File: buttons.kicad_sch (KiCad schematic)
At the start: 21 parts, among them SW1 SW_SPST, SW10 SW_SPST, SW11 SW_SPST, SW12 SW_SPST, SW13 SW_SPST, SW14 SW_SPST, SW15 SW_SPST, SW16 SW_SPST, SW17 SW_SPST, SW18 SW_SPST, SW19 SW_SPST, SW2 SW_SPST, SW20 SW_SPST, SW3 SW_SPST, SW4 SW_SPST, SW5 SW_SPST, SW6 SW_SPST, SW7 SW_SPST, SW8 SW_SPST, SW9 SW_SPST, U3 CD74HC4067M96

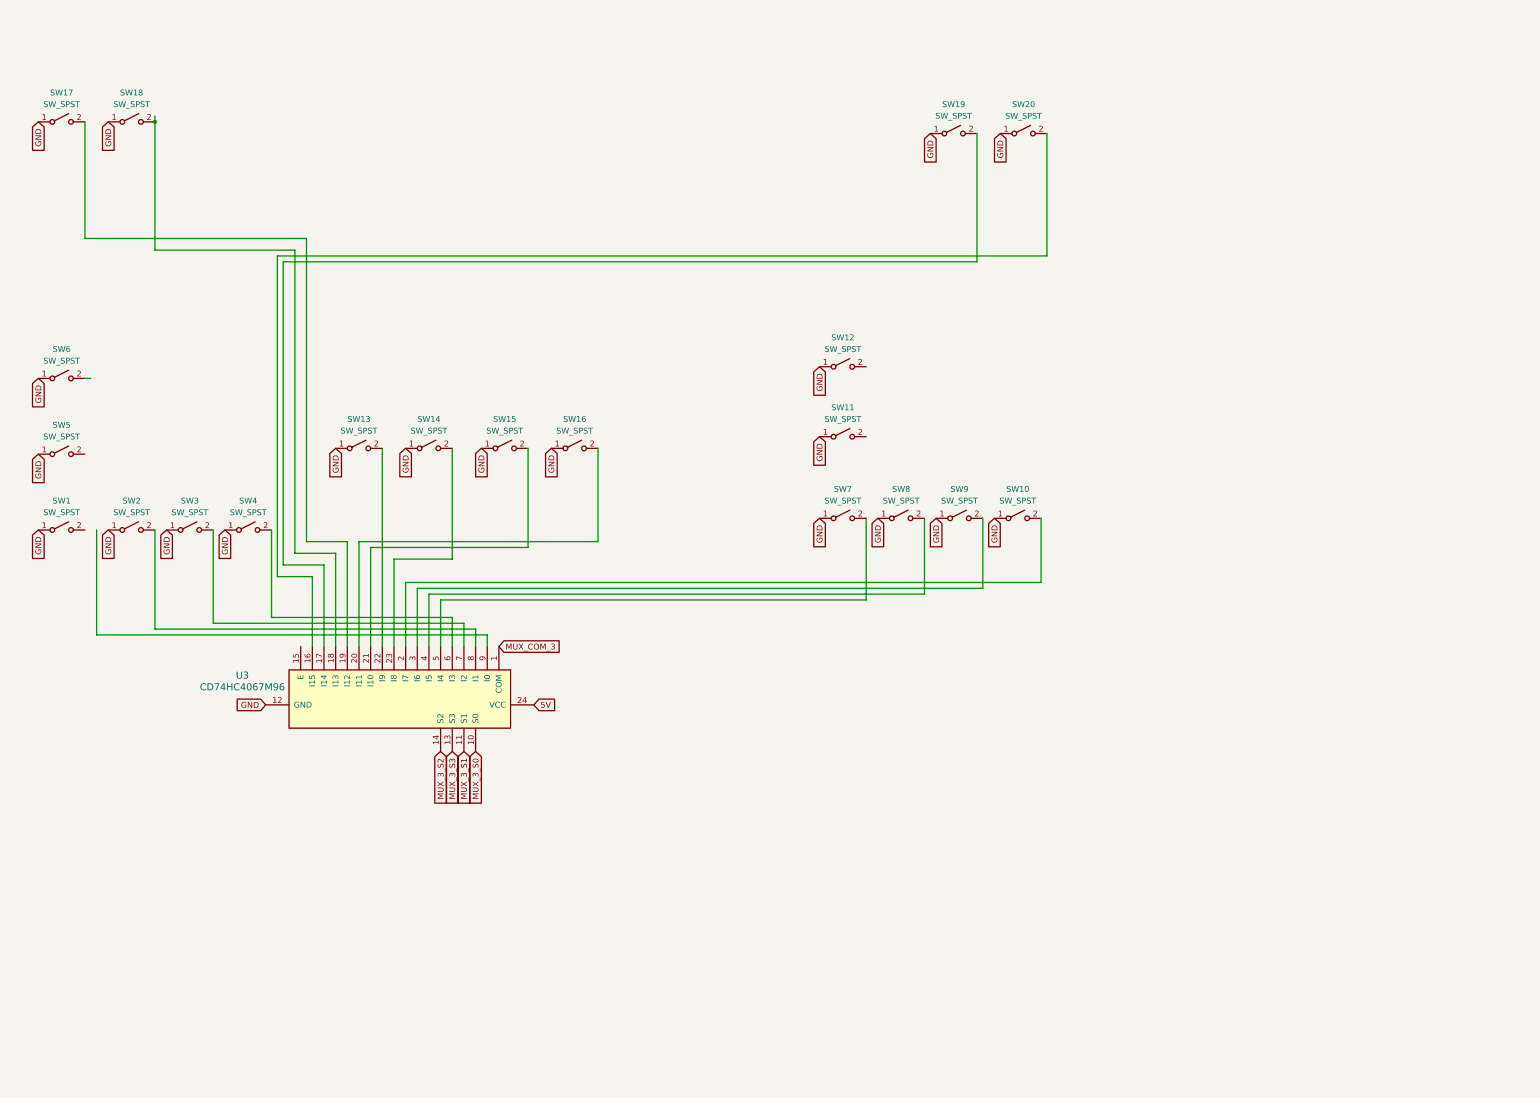
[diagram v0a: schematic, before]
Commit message: Add files via upload
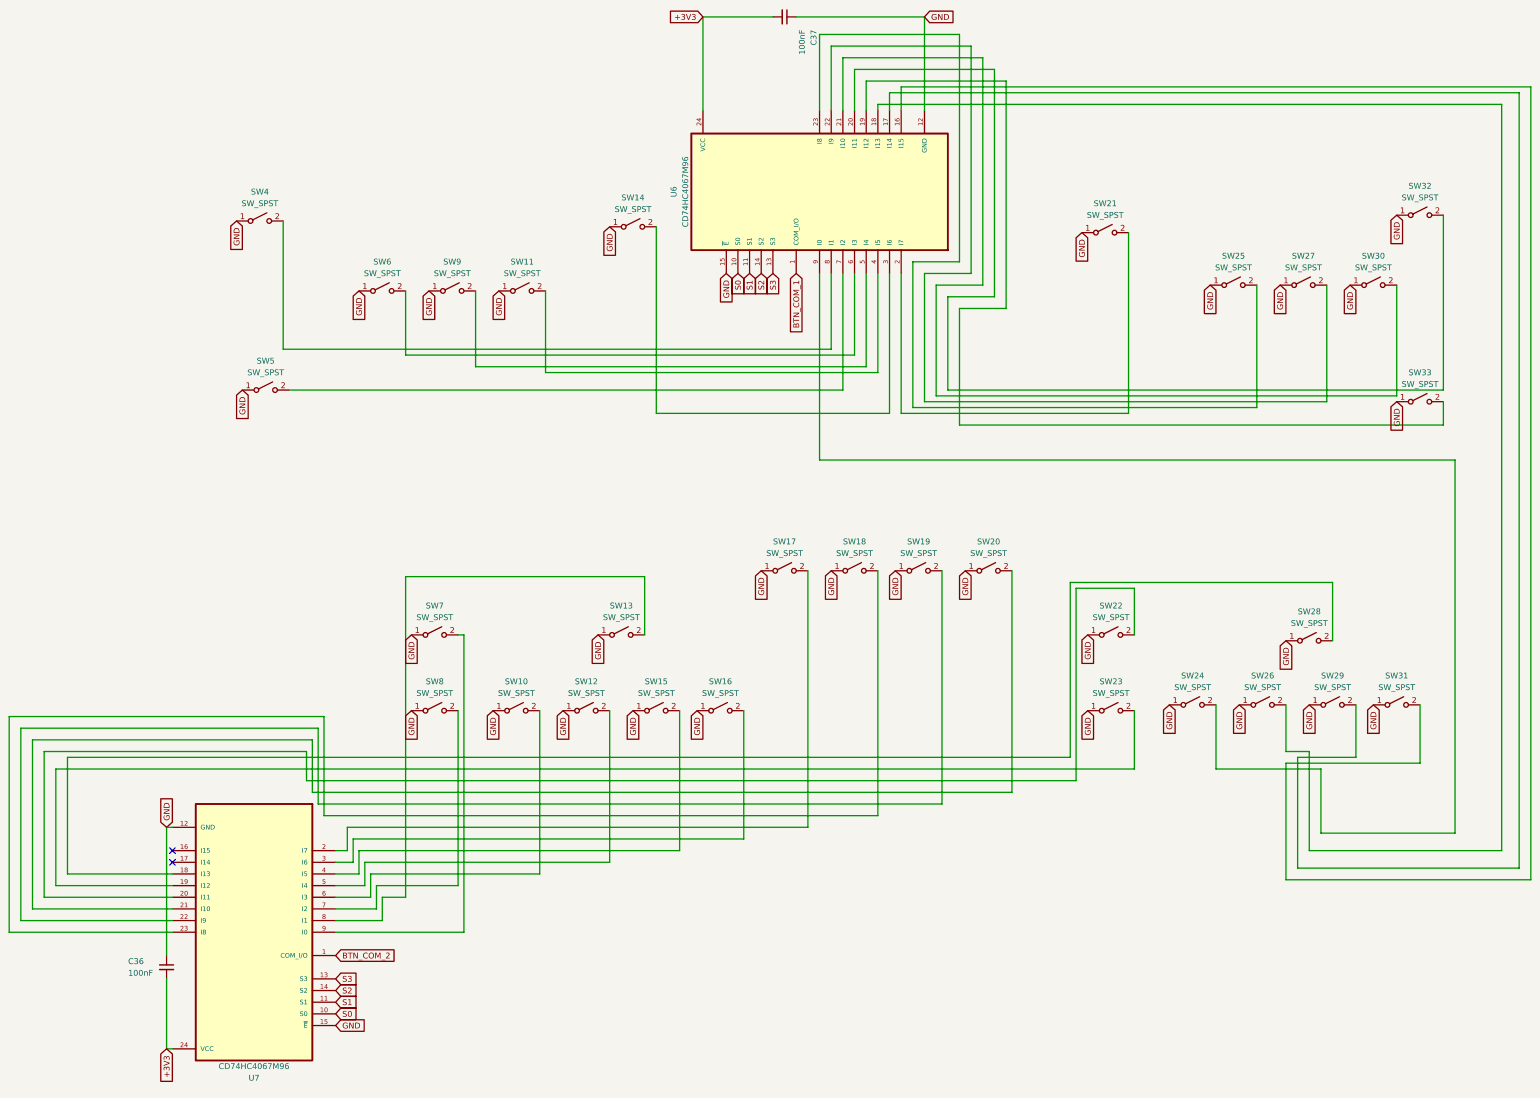
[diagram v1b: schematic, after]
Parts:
- removed SW1, SW2, SW3: SW_SPST, symbol Switch:SW_SPST
- removed U3: CD74HC4067M96, digikey-footprints:SOIC-24_W7.50mm, symbol dk_Interface-Analog-Switches-Multiplexers-Demultiplexers:CD74HC4067M96
- added C36, C37: 100nF, Capacitor_SMD:C_0603_1608Metric, symbol Device:C_Small
- added SW21, SW22, SW23, SW25, SW27, SW28, SW30, SW32, SW33: SW_SPST, TS-1088-AR02016(1):SW_TS-1088-AR02016, symbol Switch:SW_SPST
- added SW24, SW26, SW29, SW31: SW_SPST, siliconebutton:BUTTONPAD-1x1, symbol Switch:SW_SPST
- added U6, U7: CD74HC4067M96, CD74HC4067M96:SOIC127P1030X265-24N, symbol CD74HC4067M96:CD74HC4067M96
- SW10, SW12, SW15, SW16: footprint (none) -> siliconebutton:BUTTONPAD-1x1
- SW11, SW13, SW14, SW17, SW18, SW19, SW20, SW4, SW5, SW6, SW7, SW8, SW9: footprint (none) -> TS-1088-AR02016(1):SW_TS-1088-AR02016
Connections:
- net GND: now also C36.1, C37.1, SW21.1 (A), SW22.1 (A), SW23.1 (A), SW24.1 (A), SW25.1 (A), SW26.1 (A), SW27.1 (A), SW28.1 (A), SW29.1 (A), SW30.1 (A), SW31.1 (A), SW32.1 (A), SW33.1 (A), U6.12 (GND), U6.15 (~{E}), U7.12 (GND), U7.15 (~{E})
- net at SW4.2 (B): now also U6.8 (I1)
- net at SW16.2 (B): now also U7.3 (I6)
- net at SW18.2 (B): now also U7.23 (I8)
- net at SW13.2 (B): now also U7.8 (I1)
- net at SW14.2 (B): now also U6.3 (I6)
- net at SW6.2 (B): now also U6.6 (I3)
- net at SW15.2 (B): now also U7.4 (I5)
- net at SW20.2 (B): now also U7.21 (I10)
- net at SW10.2 (B): now also U7.6 (I3)
- net at SW8.2 (B): now also U7.7 (I2)
- net at SW9.2 (B): now also U6.5 (I4)
- net at SW7.2 (B): now also U7.9 (I0)
- net at SW19.2 (B): now also U7.22 (I9)
- net at SW17.2 (B): now also U7.2 (I7)
- net at SW12.2 (B): now also U7.5 (I4)
- net at SW11.2 (B): now also U6.4 (I5)
- net at SW5.2 (B): now also U6.7 (I2)
- new net: SW28.2 (B), U7.18 (I13)
- new net: SW29.2 (B), U6.17 (I14)
- new net: SW22.2 (B), U7.20 (I11)
- new net: SW24.2 (B), U6.9 (I0)
- new net: SW33.2 (B), U6.19 (I12)
- new net: SW27.2 (B), U6.22 (I9)
- new net: SW26.2 (B), U6.18 (I13)
- new net: SW23.2 (B), U7.19 (I12)
- new net: SW31.2 (B), U6.16 (I15)
- new net: SW32.2 (B), U6.20 (I11)
- new net: SW25.2 (B), U6.23 (I8)
- new net: SW30.2 (B), U6.21 (I10)
- new net: SW21.2 (B), U6.2 (I7)
- new net +3V3: C36.2, C37.2, U6.24 (VCC), U7.24 (VCC)
- new net BTN_COM_1: U6.1 (COM_I/O)
- new net BTN_COM_2: U7.1 (COM_I/O)
- new net S0: U6.10 (S0), U7.10 (S0)
- new net S1: U6.11 (S1), U7.11 (S1)
- new net S2: U6.14 (S2), U7.14 (S2)
- new net S3: U6.13 (S3), U7.13 (S3)
- no-connect marks 0 -> 2
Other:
- company: Alex Goldberg -> Alex G
- title: MiniMixer -> @opensourcedj on twitter
